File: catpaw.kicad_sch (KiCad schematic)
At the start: 36 parts, among them J1 Conn_01x01_Socket_red, J2 Conn_01x01_Socket_black, J3 m12,Acode,5pin,femalesocket (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, J4 m8, 4Pin Supply Connector FEM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, J5 m8, 4Pin Supply Connector Bec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, J6 m12,Acode,5pin,femalesocket B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, J7 m12,Acode,5pin,femalesocket C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, SW1 SW_DPST, U1 INA826, U2 ${SIM.PARAMS}

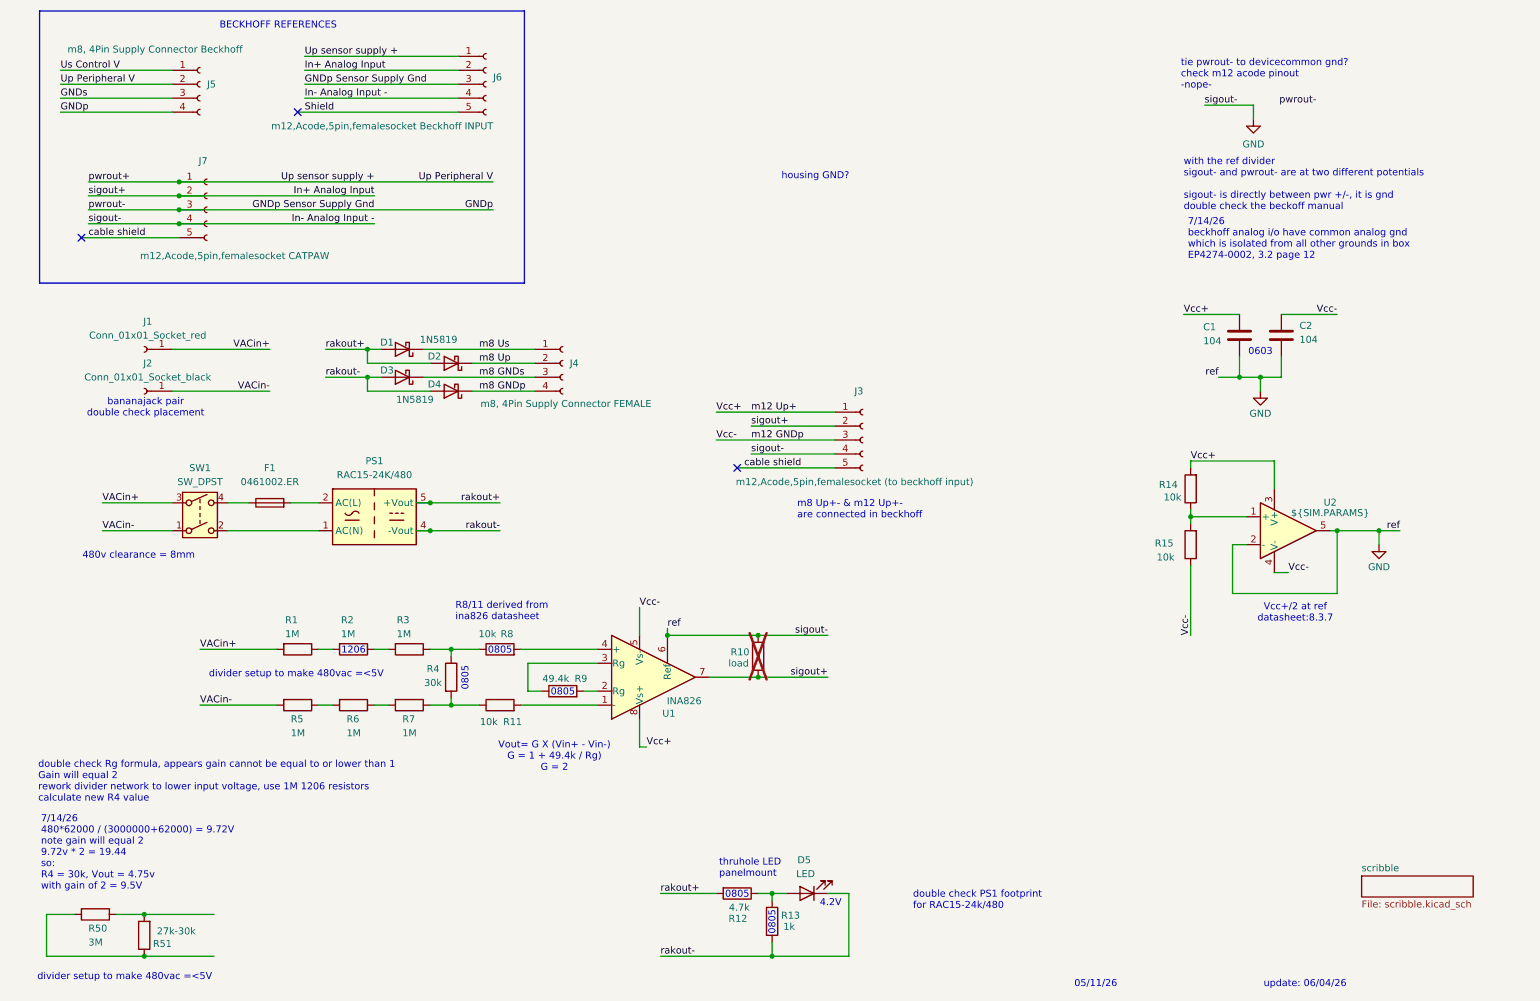
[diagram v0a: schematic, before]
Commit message: end of day
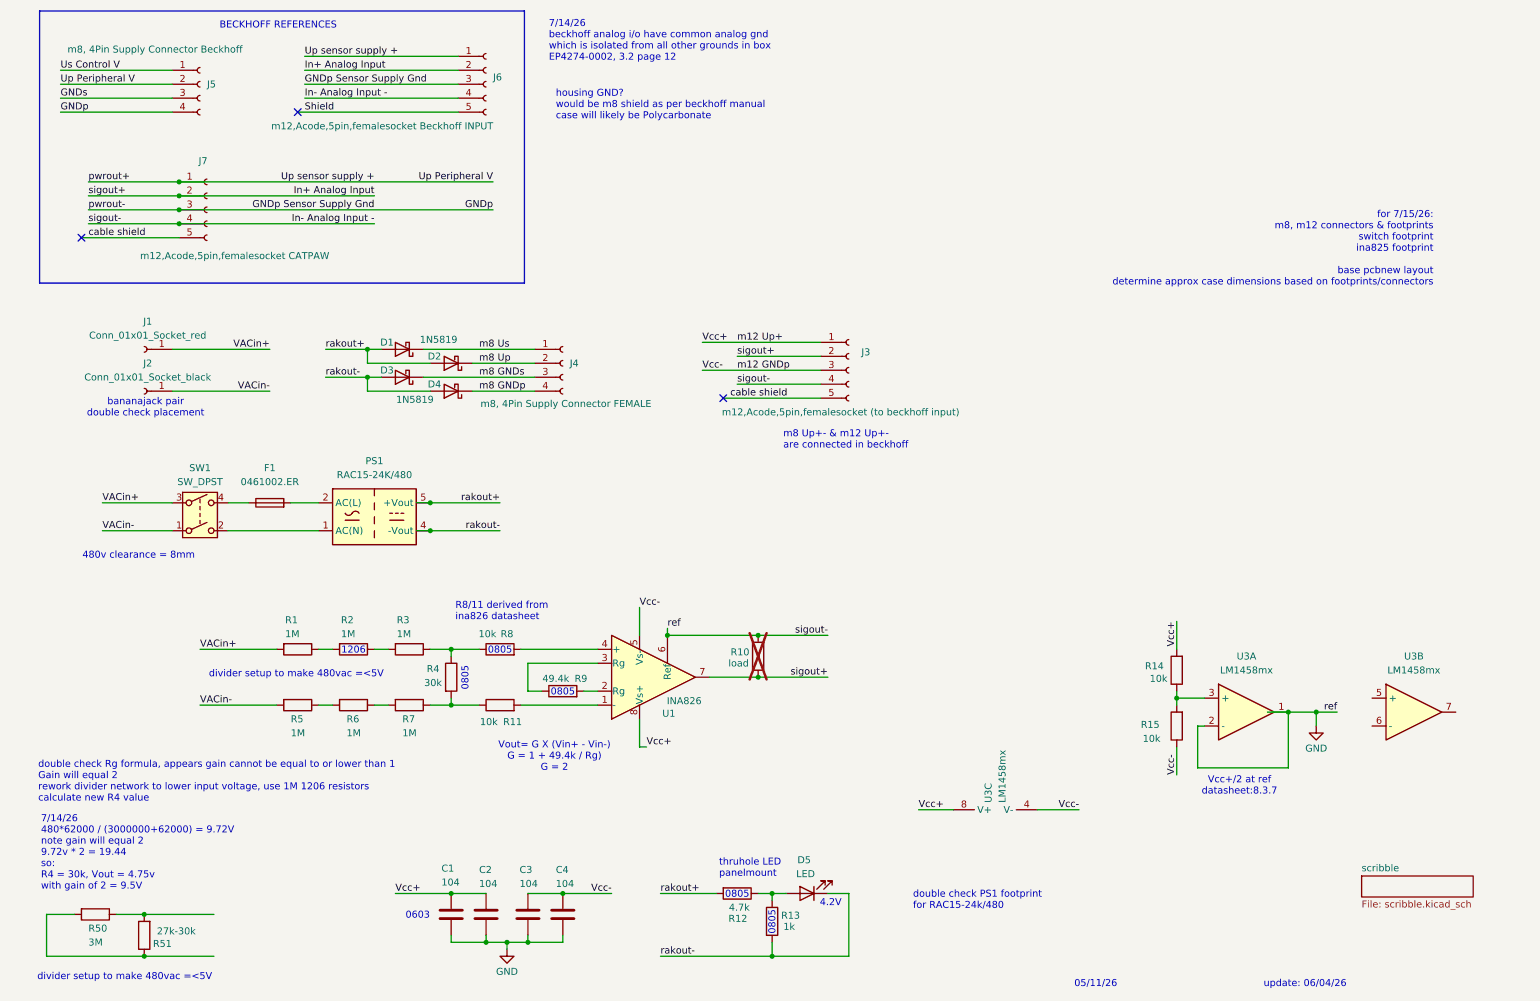
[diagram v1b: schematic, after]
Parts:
- removed U2: ${SIM.PARAMS}, symbol Simulation_SPICE:OPAMP
- added C3, C4: 104, 0603, symbol Device:C
- added U3: LM1458mx, Package_SO:SOIC-8_3.9x4.9mm_P1.27mm, symbol Device:Opamp_Dual
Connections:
- net GND: now also C3.1, C4.1, U3.1, U3.2 (-)
- net Vcc+: now also C2.2, U3.8 (V+)
- net Vcc-: now also C3.2, C4.2, U3.4 (V-); no longer C2.2
- net at R14.1, R15.2: now also U3.3 (+)
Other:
- note added: "for 7/15/26: m8, m12 connectors & footprints switch footprint ina825 footprint base pcbnew layout determine approx case dimensions based on footprints/connectors"
- note added: "housing GND? would be m8 shield as per beckhoff manual case will likely be Polycarbonate"
- note removed: "housing GND?"
- note removed: "tie pwrout- to devicecommon gnd? check m12 acode pinout -nope-"
- note removed: "with the ref divider sigout- and pwrout- are at two different potentials sigout- is directly between pwr +/-, it is gnd double check the beckoff manual"
- moved on the sheet: C1, C2, J3, R14, R15
